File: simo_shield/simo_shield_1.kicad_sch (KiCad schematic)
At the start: 8 parts, among them J1 modulo_usb_debug, J2 conector_bateria, U1 modulo_flash_externa, U2 elemon_board, U3 bluepill_board_stm32, U4 modulo_acelerometro

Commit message: update en simo_bateria
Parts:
- J2: footprint Connector_JST:JST_EH_B2B-EH-A_1x02_P2.50mm_Vertical -> simo_shield:JST_EH_B2B-EH-A_1x02_P2.50mm_Vertical
- U1: footprint simo_board:conector_flash_ext -> simo_shield:conector_flash_ext
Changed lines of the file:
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@@
     (property "Reference" "U1" (id 0) (at 35.56 151.257 0))
     (property "Value" "modulo_flash_externa" (id 1) (at 35.56 153.797 0))
-    (property "Footprint" "simo_board:conector_flash_ext" (id 2) (at 48.26 156.972 0)
+    (property "Footprint" "simo_shield:conector_flash_ext" (id 2) (at 48.26 156.972 0)
       (effects (font (size 1.27 1.27)) hide)
     )
@@
       (effects (font (size 1.27 1.27)) (justify left))
     )
-    (property "Footprint" "Connector_JST:JST_EH_B2B-EH-A_1x02_P2.50mm_Vertical" (id 2) (at 243.967 108.458 0)
+    (property "Footprint" "simo_shield:JST_EH_B2B-EH-A_1x02_P2.50mm_Vertical" (id 2) (at 243.967 108.458 0)
       (effects (font (size 1.27 1.27)) hide)
     )
@@
     )
     (path "/aa8a4ce4-263f-4980-8d9f-4f0f7a62a8f5"
-      (reference "J2") (unit 1) (value "conector_bateria") (footprint "Connector_JST:JST_EH_B2B-EH-A_1x02_P2.50mm_Vertical")
+      (reference "J2") (unit 1) (value "conector_bateria") (footprint "simo_shield:JST_EH_B2B-EH-A_1x02_P2.50mm_Vertical")
     )
     (path "/50ab3c25-18ac-4348-9b10-e46fc412d281"
-      (reference "U1") (unit 1) (value "modulo_flash_externa") (footprint "simo_board:conector_flash_ext")
+      (reference "U1") (unit 1) (value "modulo_flash_externa") (footprint "simo_shield:conector_flash_ext")
     )
     (path "/4e546ac2-24a9-4fe8-8ba3-1b8a7c4f035f"

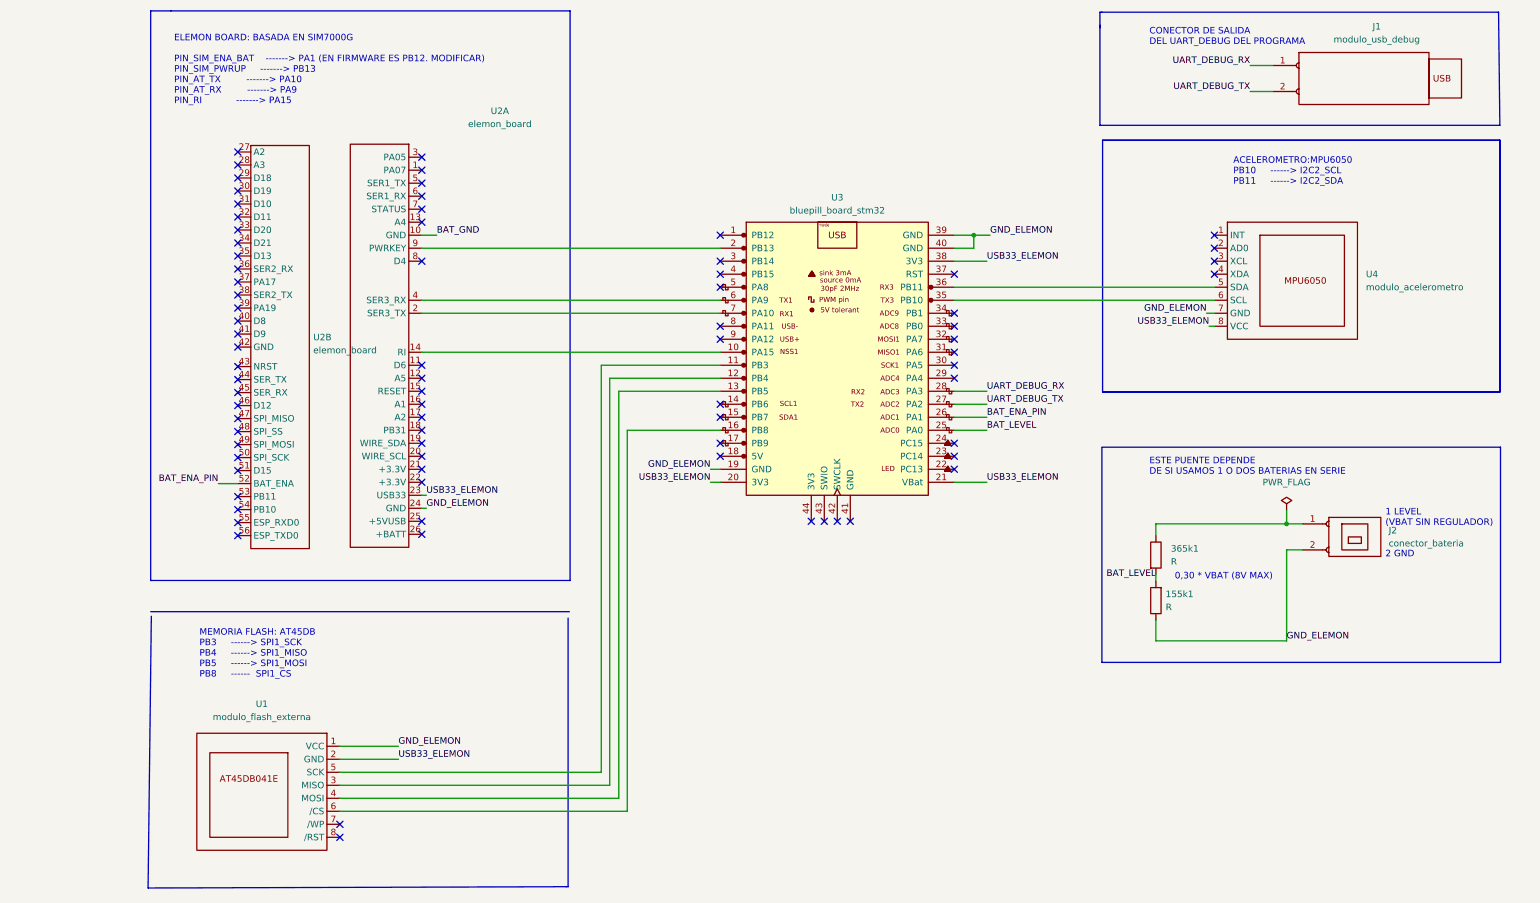
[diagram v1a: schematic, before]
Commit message: update en ambas placas, revision 02
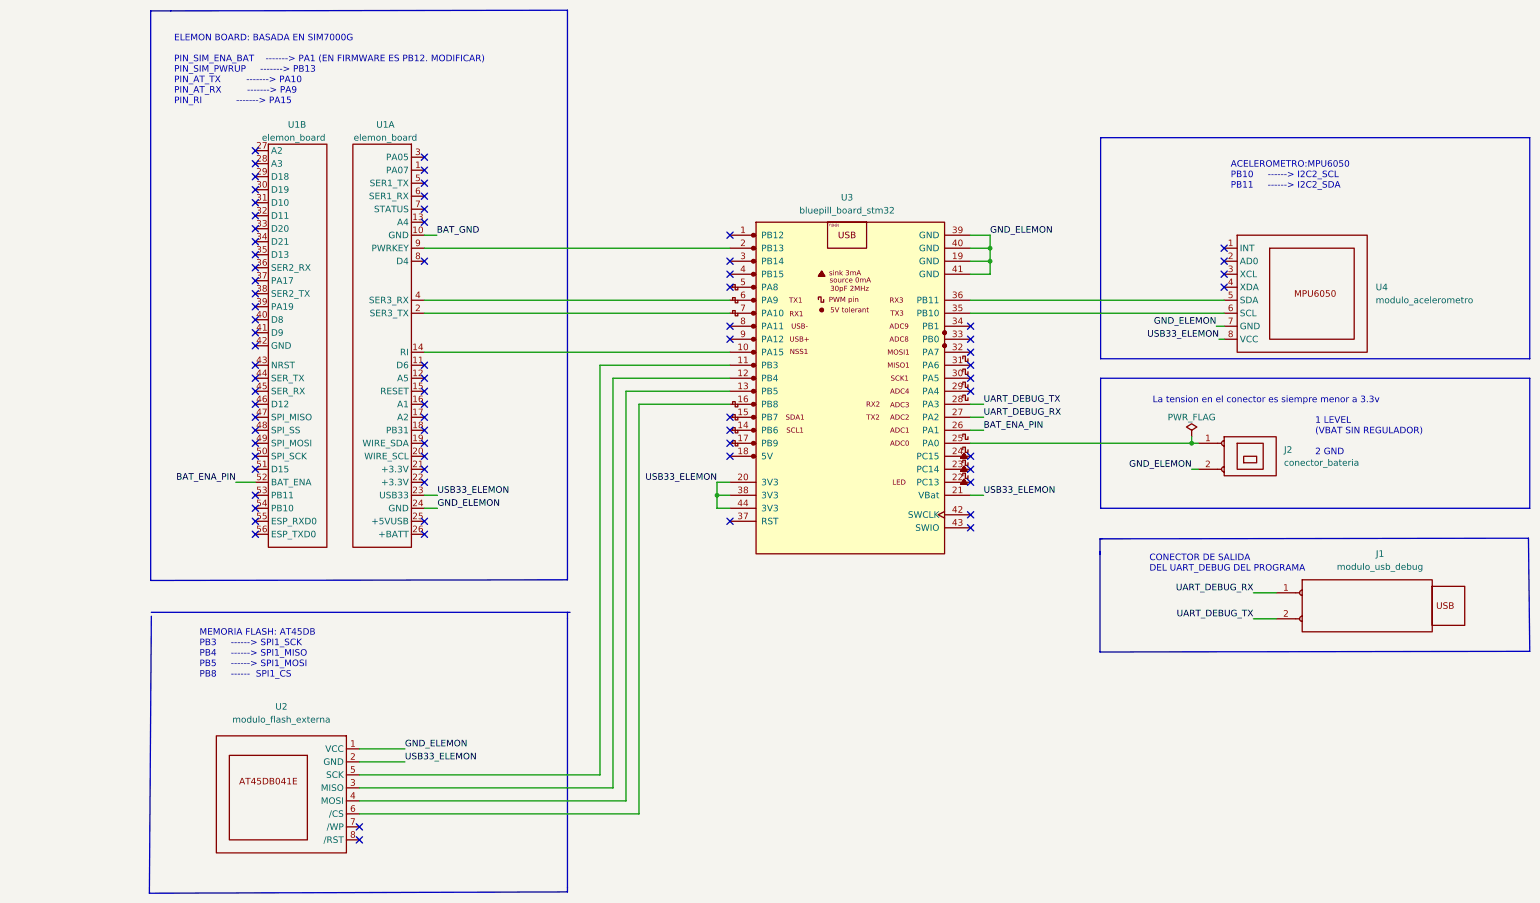
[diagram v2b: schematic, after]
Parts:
- removed 155k1, 365k1: R, simo_shield:R_0805_2012Metric, symbol simo_shield:R
- removed U2: elemon_board, simo_shield:elemon_board, symbol simo_shield:elemon_board
- added U1: elemon_board, simo_shield:elemon_board, symbol simo_shield:elemon_board
- renumbered U1 to U2
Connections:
- net BAT_LEVEL is gone; now on an unnamed net: U3.25 (PA0)
- net BAT_ENA_PIN: now also U1.52 (BAT_ENA)
- net BAT_GND: now also U1.10 (GND)
- net GND_ELEMON: now also U3.41 (GND), U1.24 (GND)
- net UART_DEBUG_RX: now also U3.27 (PA2); no longer U3.28 (PA3)
- net UART_DEBUG_TX: now also U3.28 (PA3); no longer U3.27 (PA2)
- net USB33_ELEMON: now also U3.44 (3V3), U1.23 (USB33)
- net at U3.10 (PA15): now also U1.14 (RI)
- net at U3.7 (PA10): now also U1.2 (SER3_TX)
- net at U3.6 (PA9): now also U1.4 (SER3_RX)
- net at U3.2 (PB13): now also U1.9 (PWRKEY)
- no-connect marks 78 -> 76
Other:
- note added: "La tension en el conector es siempre menor a 3.3v"
- note removed: "0,30 * VBAT (8V MAX)"
- note removed: "ESTE PUENTE DEPENDE DE SI USAMOS 1 O DOS BATERIAS EN SERIE"
- moved on the sheet: J1, J2, U2, U3, U4
